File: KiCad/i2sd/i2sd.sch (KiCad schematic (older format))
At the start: 21 parts, among them IC1 ATMEGA8-AI, P1 CONN_4, P2 CONN_4, P3 CONN_4, SW1 SW_PUSH, U1 MCP_1700, X1 CRYSTAL

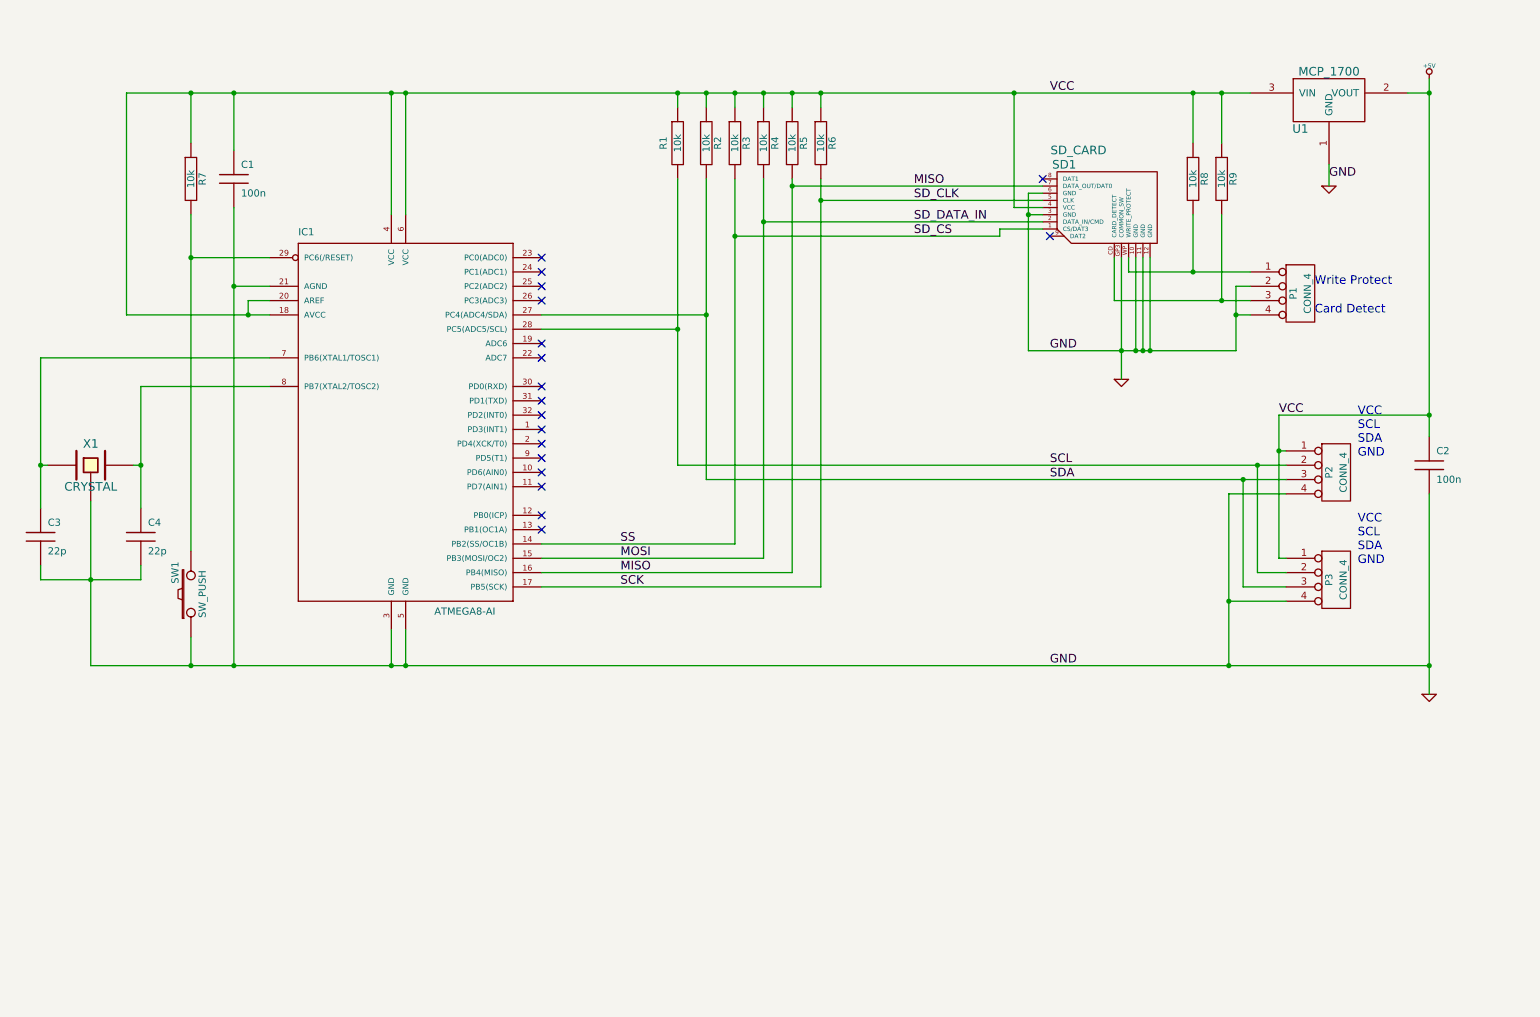
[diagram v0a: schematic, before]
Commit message: 2011-05-12 : i2sd : Schematic and PCB
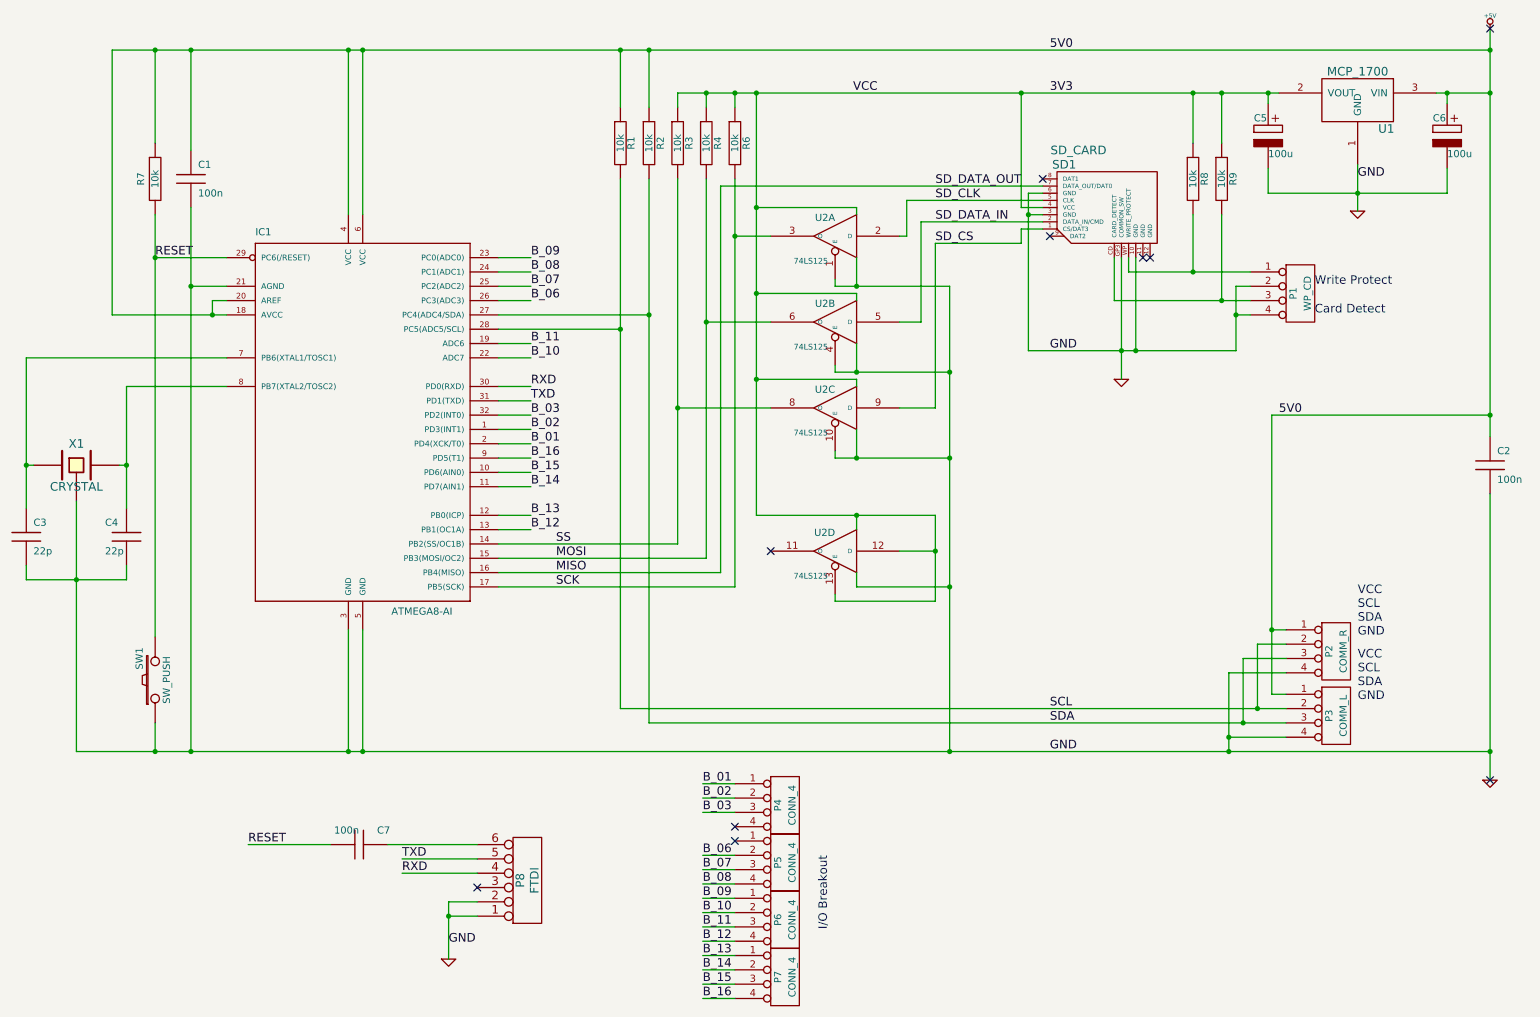
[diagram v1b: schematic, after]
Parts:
- removed R5: 10k, symbol R
- added C5, C6: 100u, CP_5x11mm, symbol C_POL
- added C7: 100n, C2, symbol C
- added P4, P5, P6, P7: CONN_4, pin_strip_4, symbol CONN_4
- added P8: FTDI, pin_strip_6-90, symbol CONN_6
- added U2: 74LS125, SO14E, symbol 74LS125
- C1, C2: footprint (none) -> C2
- C3, C4: footprint (none) -> C1
- P1: value CONN_4 -> WP_CD; footprint (none) -> pin_strip_4
- P2: value CONN_4 -> COMM_R; footprint (none) -> pin_strip_4
- P3: value CONN_4 -> COMM_L; footprint (none) -> pin_strip_4
- R1, R2, R3, R4, R6, R7, R8, R9: footprint (none) -> R1
- SD1: footprint (none) -> Memory_Card_SD_3M
- SW1: footprint (none) -> SW-PB
- U1: footprint (none) -> SOT23-5
- X1: footprint (none) -> XTAL
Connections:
- net +5V: now also C6.1; no longer R3.1, R4.1, R6.1, R8.1, R9.1, SD1.4 (VCC), U1.2 (VOUT)
- net GND: now also C5.2, C6.2, P8.1, P8.2, U2.1 (E), U2.10 (E), U2.4 (E), U2.7 (GND), U2.7 (GND), U2.7 (GND), U2.7 (GND); no longer SD1.11 (GND), SD1.12 (GND)
- net MOSI: now also U2.6 (O); no longer SD1.2 (DATA_IN/CMD)
- net SCK: now also U2.3 (O); no longer SD1.5 (CLK)
- net SD_CS: now also U2.9 (D); no longer IC1.14 (PB2(SS/OC1B)), R3.2
- net B_02: now reaches IC1.1 (PD3(INT1))
- net B_02: now also P4.2 (P2)
- net B_15: now reaches IC1.10 (PD6(AIN0))
- net B_15: now also P7.3 (P3)
- net B_14: now reaches IC1.11 (PD7(AIN1))
- net B_14: now also P7.2 (P2)
- net B_13: now reaches IC1.12 (PB0(ICP))
- net B_13: now also P7.1 (P1)
- net B_12: now reaches IC1.13 (PB1(OC1A))
- net B_12: now also P6.4 (P4)
- net B_11: now reaches IC1.19 (ADC6)
- net B_11: now also P6.3 (P3)
- net B_01: now reaches IC1.2 (PD4(XCK/T0))
- net B_01: now also P4.1 (P1)
- net B_10: now reaches IC1.22 (ADC7)
- net B_10: now also P6.2 (P2)
- net B_09: now reaches IC1.23 (PC0(ADC0))
- net B_09: now also P6.1 (P1)
- net B_08: now reaches IC1.24 (PC1(ADC1))
- net B_08: now also P5.4 (P4)
- net B_07: now reaches IC1.25 (PC2(ADC2))
- net B_07: now also P5.3 (P3)
- net B_06: now reaches IC1.26 (PC3(ADC3))
- net B_06: now also P5.2 (P2)
- net RESET: now reaches IC1.29 (PC6(/RESET)), R7.2, SW1.2
- net RESET: now also C7.2
- net RXD: now reaches IC1.30 (PD0(RXD))
- net RXD: now also P8.4
- net TXD: now reaches IC1.31 (PD1(TXD))
- net TXD: now also P8.5
- net B_03: now reaches IC1.32 (PD2(INT0))
- net B_03: now also P4.3 (P3)
- net B_16: now reaches IC1.9 (PD5(T1))
- net B_16: now also P7.4 (P4)
- new net: C7.1, P8.6
- new net SD_CLK: SD1.5 (CLK), U2.2 (D)
- new net SD_DATA_IN: SD1.2 (DATA_IN/CMD), U2.5 (D)
- new net SS: IC1.14 (PB2(SS/OC1B)), R3.2, U2.8 (O)
- new net VCC: C5.1, R3.1, R4.1, R6.1, R8.1, R9.1, SD1.4 (VCC), U1.2 (VOUT), U2.12 (D), U2.13 (E), U2.14 (VCC), U2.14 (VCC), U2.14 (VCC), U2.14 (VCC)
- no-connect marks 18 -> 10
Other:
- note added: "I/O Breakout"
- moved on the sheet: C1, C2, C3, C4, IC1, P2, P3, R1, R2, R3, R4, R6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
